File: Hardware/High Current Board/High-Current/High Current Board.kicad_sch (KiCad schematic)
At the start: 37 parts, among them J1 8P8C_Shielded, J2 Conn_01x04, J3 GND, J4 Load Resistors Return, J5 +46V from Fuel Cell, K1 G2RL-1A-E, K2 G2RL-1A-E, Q1 NMOS_Substrate, Q2 NMOS, U1 TC4421AVAT, U3 HO 25-P

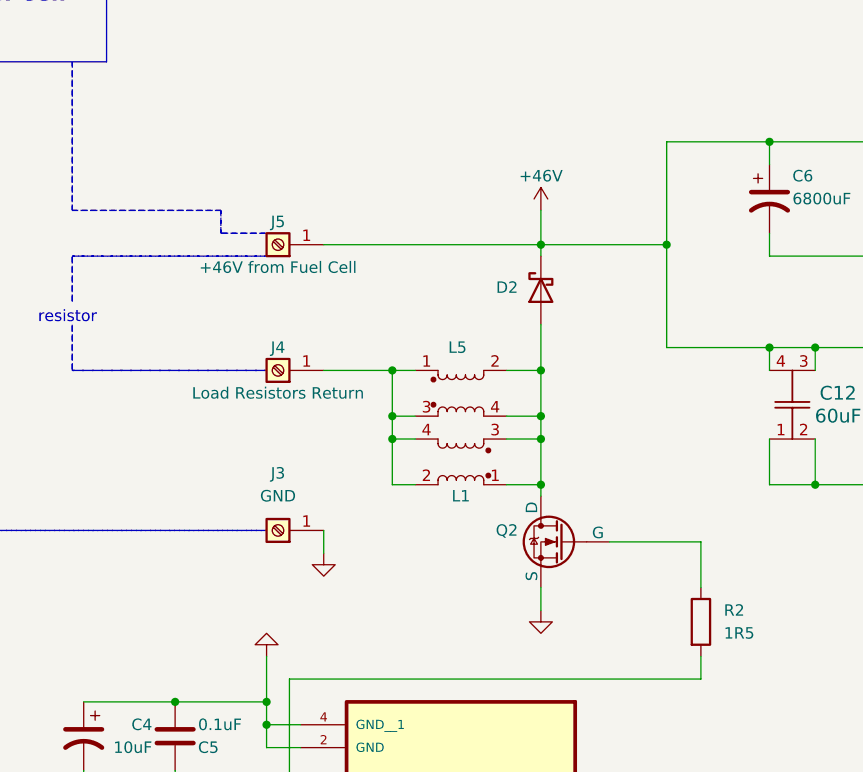
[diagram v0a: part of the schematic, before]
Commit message: PCB Update 1.0
Needs a Revision Check and we good
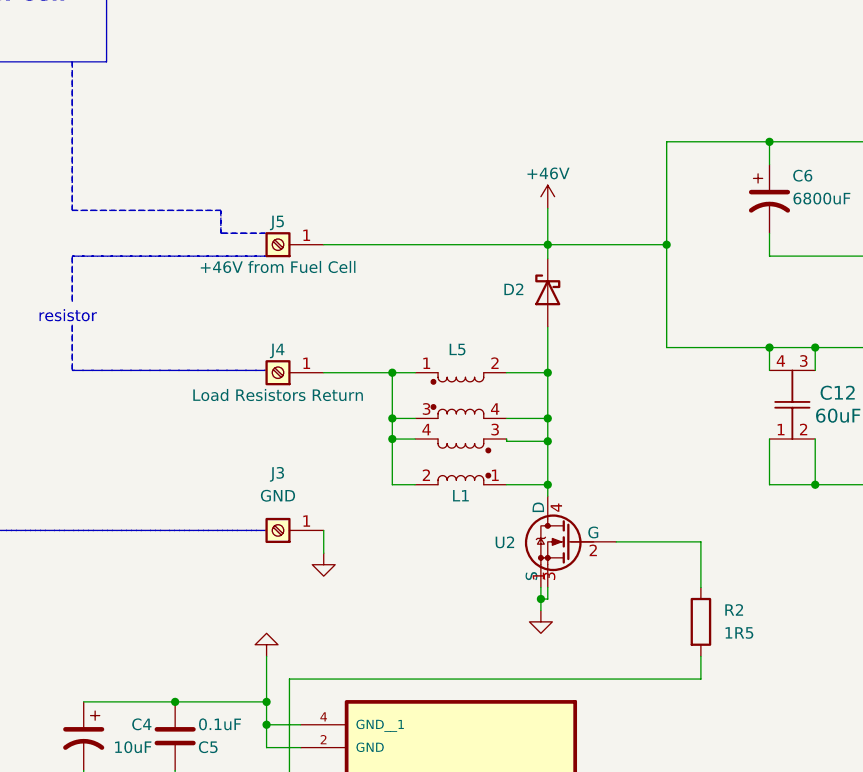
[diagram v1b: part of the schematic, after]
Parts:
- removed Q2: NMOS, filmcapacitorsfootprint:SOT-23_MCC, symbol Simulation_SPICE:NMOS
- added U2: ~, KiCADv6:GENESIC_MBR200100CTS, symbol Extra Symbols:SOT-227
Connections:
- net GND: now also U2.1 (S), U2.3 (S)
- net at D2.2 (A), L1.1, L1.3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: now also U2.4 (D)
- net at R2.1: now also U2.2 (G)
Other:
- moved on the sheet: D2
